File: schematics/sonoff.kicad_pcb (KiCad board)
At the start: 2 copper layers, 49.9 x 43.1 mm, 17 parts, among them J1 Screw_Terminal_01x04, J2 Screw_Terminal_01x04, K1 Relay_SPDT, K2 Relay_SPDT, Q1 2N7000, Q2 2N7000, U1 ESP-01v090

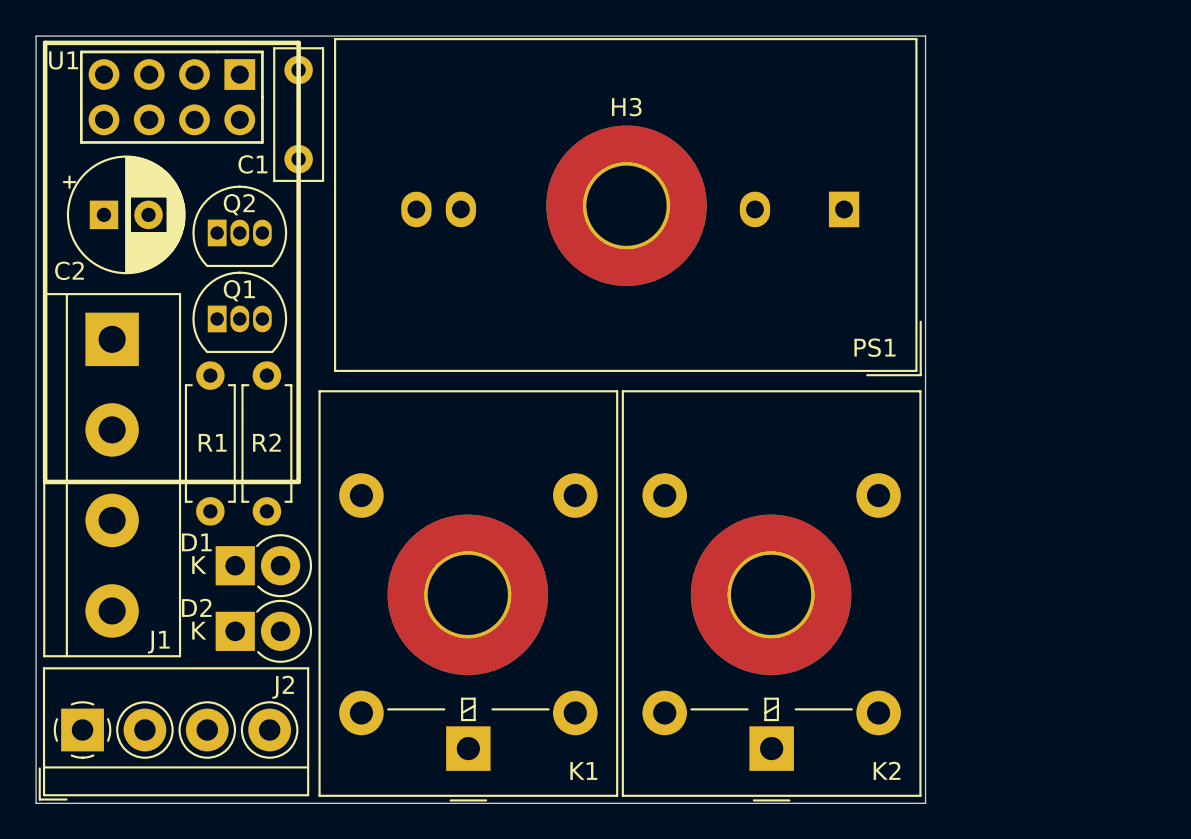
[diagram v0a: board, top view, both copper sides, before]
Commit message: chore: improved design.
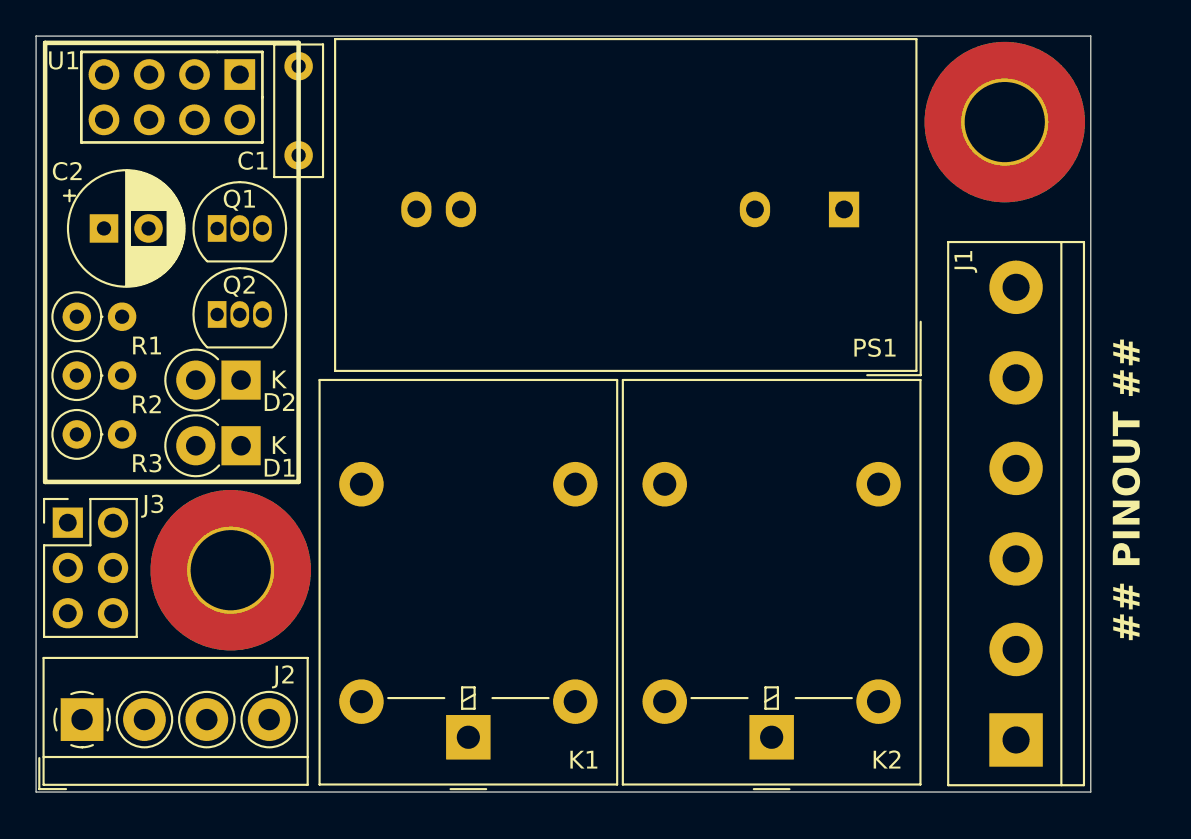
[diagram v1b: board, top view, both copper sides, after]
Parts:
- removed H3: MountingHole, MountingHole:MountingHole_4.5mm_Pad_TopBottom
- added J3: Conn_02x03_Odd_Even, Connector_PinHeader_2.54mm:PinHeader_2x03_P2.54mm_Vertical, F.Cu at (126.1, 112.3)
- added R3: R, Resistor_THT:R_Axial_DIN0207_L6.3mm_D2.5mm_P2.54mm_Vertical, F.Cu at (126.6, 107.3)
- J1: value Screw_Terminal_01x04 -> Screw_Terminal_01x06; footprint TerminalBlock:TerminalBlock_bornier-4_P5.08mm -> TerminalBlock:TerminalBlock_bornier-6_P5.08mm
- R1, R2: footprint Resistor_THT:R_Axial_DIN0207_L6.3mm_D2.5mm_P7.62mm_Horizontal -> Resistor_THT:R_Axial_DIN0207_L6.3mm_D2.5mm_P2.54mm_Vertical
- moved J1 55.5 mm to (179.3, 124.5), turned to 90 degrees
- moved H2 29.6 mm to (178.7, 89.8)
- moved D2 14.1 mm to (135.8, 104.3), turned to 180 degrees
- moved H1 13.4 mm to (135.3, 114.9)
- moved R2 10.7 mm to (126.6, 104.0), turned to 0 degrees
- moved R1 8.19 mm to (126.6, 100.7), turned to 0 degrees
- moved D1 6.74 mm to (135.8, 108.0), turned to 180 degrees
- moved C2 0.76 mm to (128.1, 95.8)
- moved K1 0.64 mm to (148.6, 124.3)
- moved K2 0.64 mm to (165.6, 124.3)
- moved J2 0.58 mm to (126.9, 123.3)
- moved Q1 0.25 mm to (134.5, 95.8)
- moved Q2 0.25 mm to (134.5, 100.6)
- moved C1 0.21 mm to (139.1, 86.7)
- renumbered Q2 to Q1, Q1 to Q2
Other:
- board size 49.9 x 43.1 mm -> 59.2 x 42.4 mm
- board text added: "## PINOUT ##"
